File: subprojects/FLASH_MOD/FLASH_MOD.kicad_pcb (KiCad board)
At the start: 2 copper layers, 14 x 22.9 mm, 10 parts, among them U1 W25Q128JVS, U101 ER-TFTM028-4

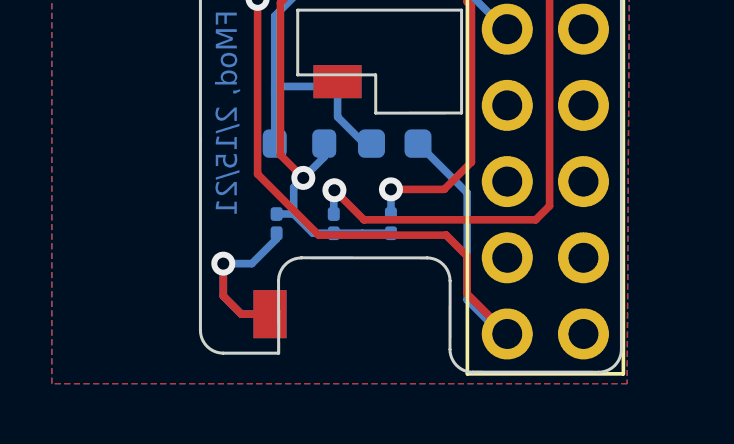
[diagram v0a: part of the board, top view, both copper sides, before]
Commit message: Flash mod add generated files
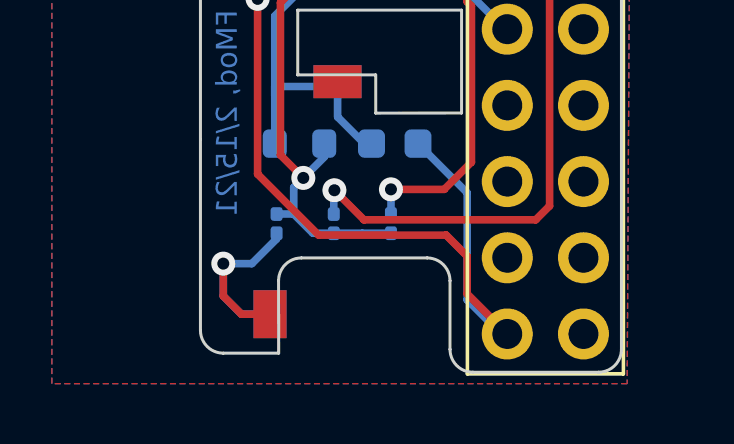
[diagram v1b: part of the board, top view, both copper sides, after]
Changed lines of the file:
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@@
     (pad 8 smd roundrect (at 3.6 1.905 90) (size 1.6 0.6) (layers B.Cu B.Paste B.Mask) (roundrect_rratio 0.25)
       (net 2 +3V3))
-    (model ${KISYS3DMOD}/Package_SO.3dshapes/SOIC-8_5.23x5.23mm_P1.27mm.wrl
-      (at (xyz 0 0 0))
-      (scale (xyz 1 1 1))
-      (rotate (xyz 0 0 0))
-    )
     (model ${KISYS3DMOD}/Package_SO.3dshapes/SOIC-8_5.275x5.275mm_P1.27mm.step
       (at (xyz 0 0 0))
@@
   (gr_line (start 205.232 88.138) (end 205.232 81.788) (layer Edge.Cuts) (width 0.1))
   (gr_line (start 207.84 88.9) (end 205.994 88.9) (layer Edge.Cuts) (width 0.1))
-  (gr_line (start 218.5035 89.535) (end 214.3125 89.53) (layer Edge.Cuts) (width 0.1))
-  (gr_line (start 212.7885 85.725) (end 208.5975 85.72) (layer Edge.Cuts) (width 0.1))
-  (gr_line (start 213.5505 88.773) (end 213.555 86.487) (layer Edge.Cuts) (width 0.1))
+  (gr_line (start 218.5035 89.535) (end 214.3125 89.535) (layer Edge.Cuts) (width 0.1))
+  (gr_line (start 212.7885 85.725) (end 208.5975 85.725) (layer Edge.Cuts) (width 0.1))
+  (gr_line (start 213.5505 88.773) (end 213.5505 86.487) (layer Edge.Cuts) (width 0.1))
   (gr_line (start 211.074 80.894) (end 211.074 79.624) (layer Edge.Cuts) (width 0.1))
   (gr_line (start 213.936 80.894) (end 211.074 80.899) (layer Edge.Cuts) (width 0.1))
